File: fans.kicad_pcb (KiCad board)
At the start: 2 copper layers, 76.2 x 25.4 mm, 18 parts, among them J1 CONN_01X02, J2 CONN_01X02, J3 CONN_01X02, J4 CONN_01X02, Q1 BC549, Q2 BC549, Q3 BC549, U1 Adafruit_Huzzah, U2 LD1117AV33

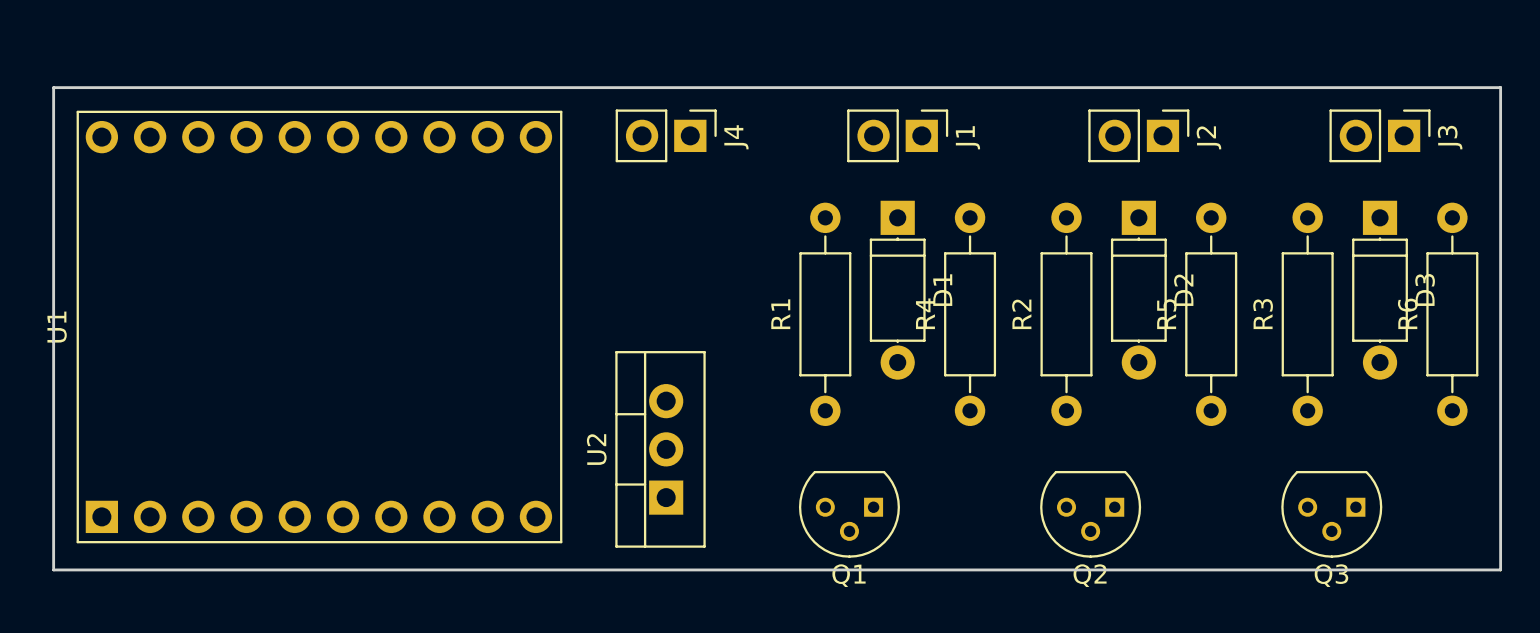
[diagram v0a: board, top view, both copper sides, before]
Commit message: First finished layout.
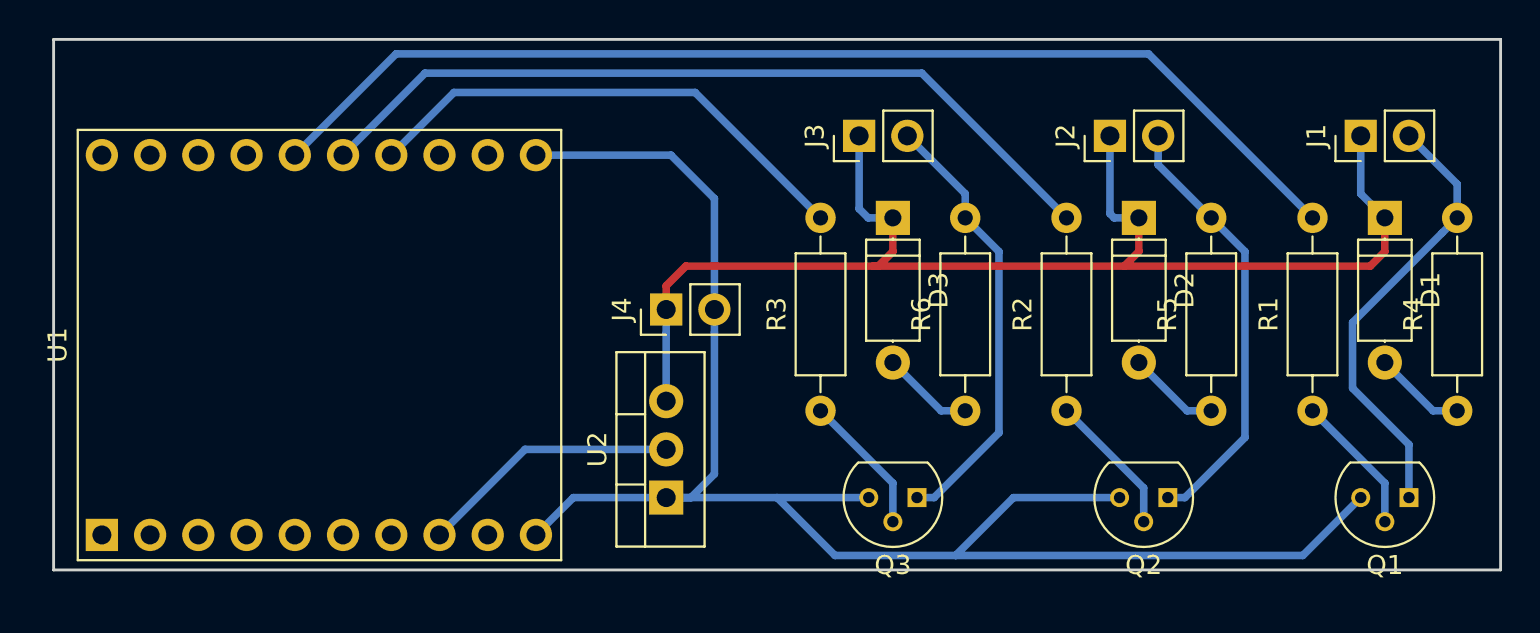
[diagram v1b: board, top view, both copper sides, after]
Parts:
- moved J3 28.7 mm to (207.5, 71.1), turned to 90 degrees
- moved Q1 28.2 mm to (236.5, 90.2)
- moved D1 25.7 mm to (235.2, 75.4)
- moved D3 25.7 mm to (209.3, 75.4)
- moved R1 25.7 mm to (231.4, 85.6)
- moved R3 25.7 mm to (205.5, 85.6)
- moved R4 25.7 mm to (239.0, 85.6)
- moved R6 25.7 mm to (213.1, 85.6)
- moved Q3 23.1 mm to (210.6, 90.2)
- moved J1 23.1 mm to (233.9, 71.1), turned to 90 degrees
- moved J4 9.23 mm to (197.4, 80.3), turned to 90 degrees
- moved Q2 2.84 mm to (223.8, 90.2)
- moved J2 2.79 mm to (220.7, 71.1), turned to 90 degrees
- moved U1 0.95 mm to (167.6, 82.1)
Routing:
- net GND: track 0.00 -> 90.1 mm
- net +12V: track 0.00 -> 68.8 mm
- net Net-(R1-Pad2): track 0.00 -> 59.4 mm
- net Net-(R2-Pad2): track 0.00 -> 43.0 mm
- net Net-(R3-Pad2): track 0.00 -> 26.7 mm
- net Net-(J1-Pad2): track 0.00 -> 23.6 mm
- net Net-(J3-Pad2): track 0.00 -> 23.4 mm
- net Net-(J2-Pad2): track 0.00 -> 23.2 mm
- net +3V3: track 0.00 -> 13.8 mm
- net Net-(Q2-Pad2): track 0.00 -> 7.53 mm
- net Net-(Q3-Pad2): track 0.00 -> 7.42 mm
- net Net-(Q1-Pad2): track 0.00 -> 7.42 mm
- net Net-(D2-Pad2): track 0.00 -> 4.86 mm
- net Net-(D1-Pad2): track 0.00 -> 4.86 mm
- net Net-(D3-Pad2): track 0.00 -> 4.86 mm
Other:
- board size 76.2 x 25.4 mm -> 76.2 x 27.9 mm
- net class Default: clearance 0.2 -> 0.4; trace_width 0.25 -> 0.4; via_dia 0.6 -> 2.5; via_drill 0.4 -> 1
- rule trace_clearance: 0.2 -> 0.4
- rule trace_min: 0.2 -> 0.4
- rule via_min_size: 0.4 -> 2.5
